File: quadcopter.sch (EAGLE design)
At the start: 61 parts, among them J1 ISP, J4 SIP-10_TH-254X10, M1 MOTOR_PADS, M2 MOTOR_PADS, M3 MOTOR_PADS, M4 MOTOR_PADS, U1 ATMEGA128RFA1, Y1 16MHz

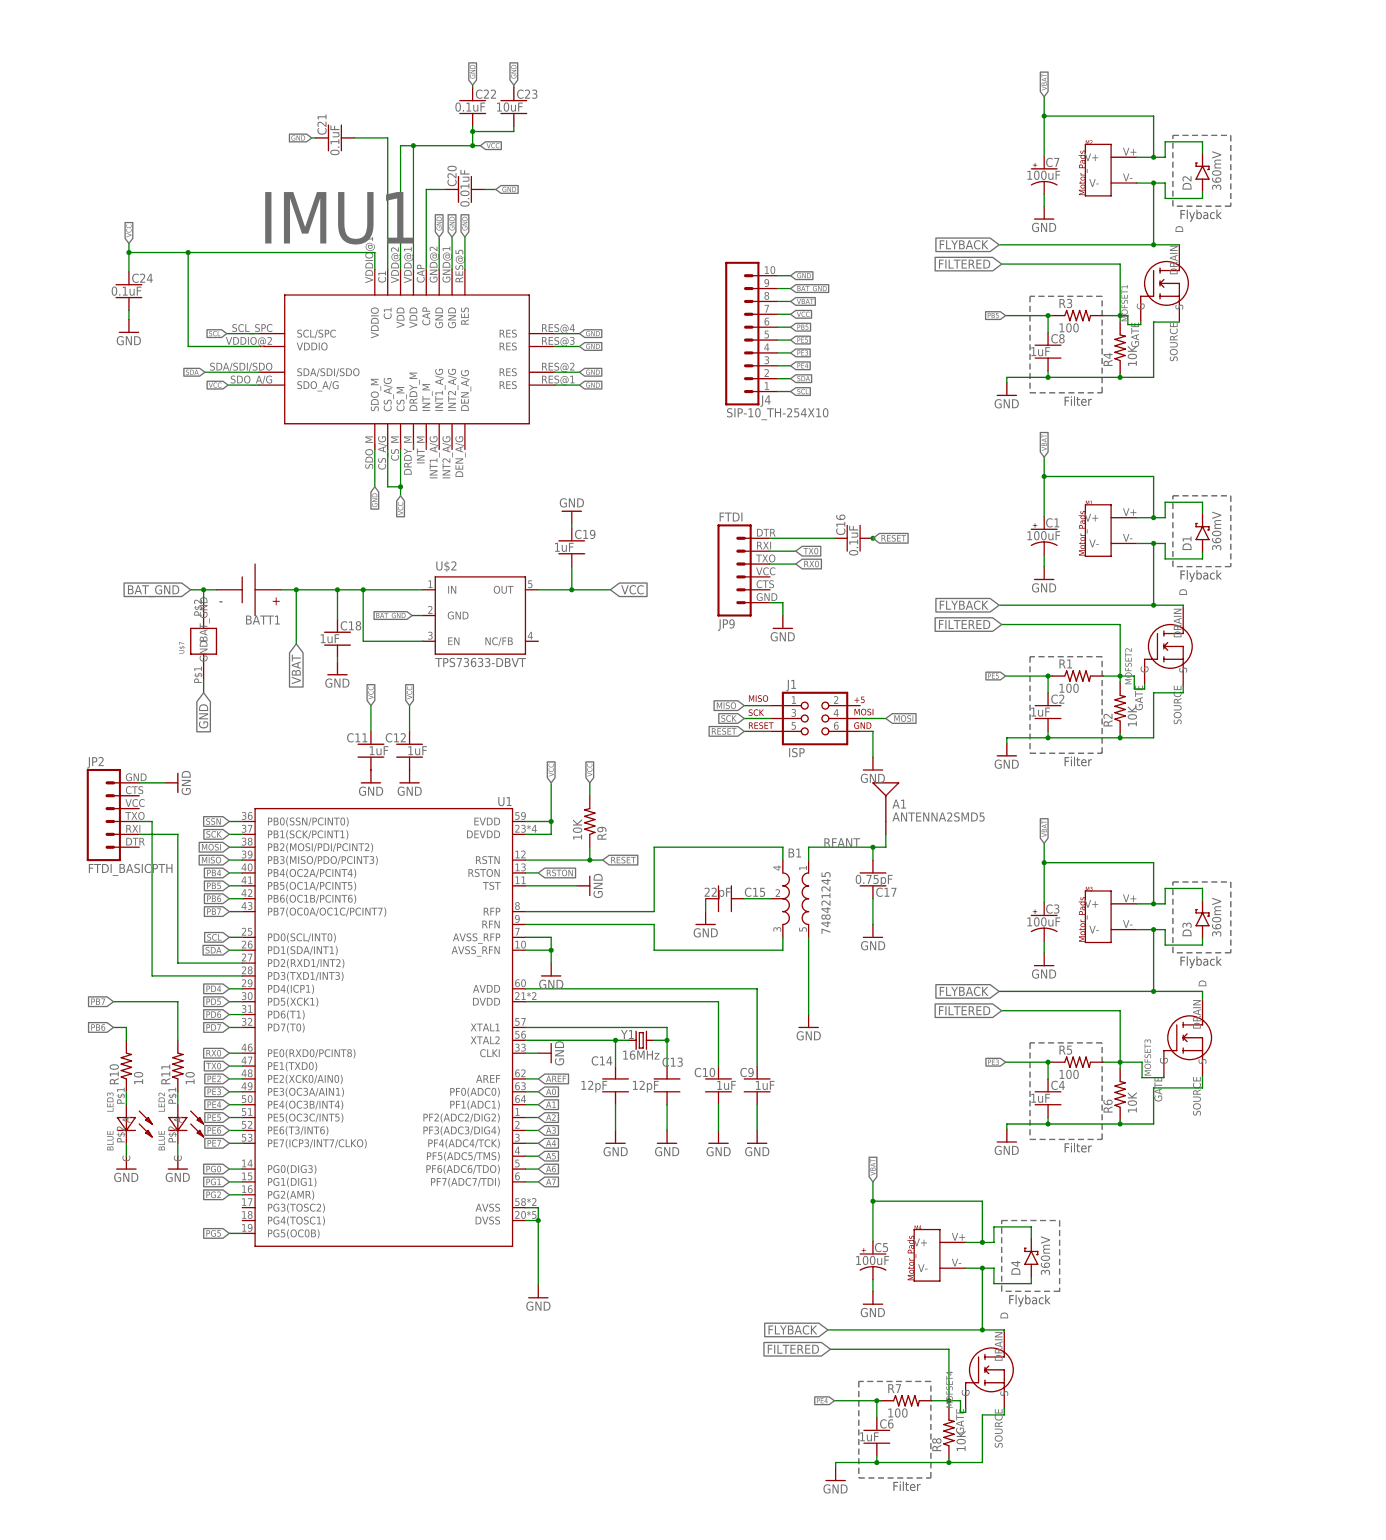
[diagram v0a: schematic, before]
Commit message: Schematic edited on April 24th
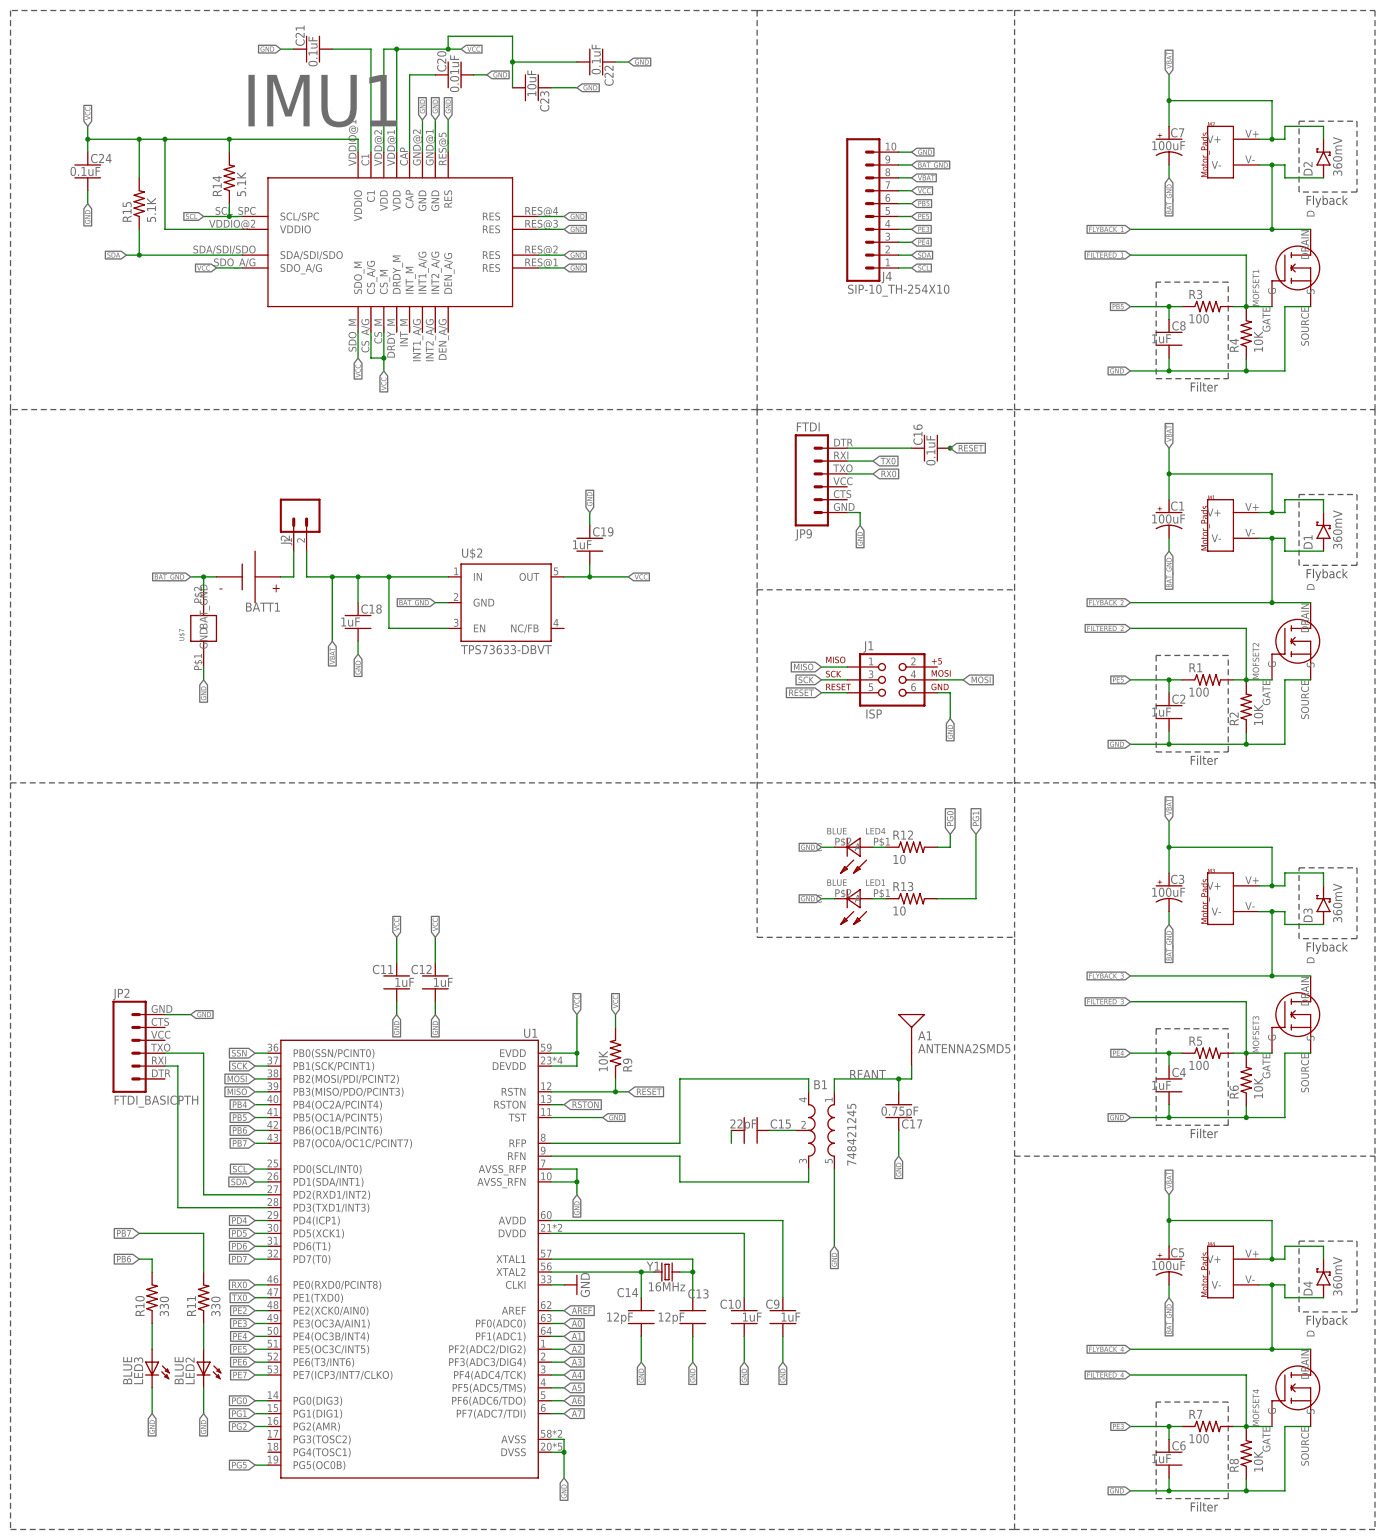
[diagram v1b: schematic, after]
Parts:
- added J2: (no value), quadparts:MALE_HEADER_2POS-2X1-0.1IN
- added LED1, LED4: BLUE, LEDs:LTST-C193TBKT-5ADISCRETE_LED
- added R12, R13: 10, quadparts_prebuilt:RESISTOR_SMD-2012-0805-10
- added R14, R15: 5.1K, quadparts_prebuilt:RESISTOR_SMD-2012-0805-5.1K
- LED2, LED3: device LEDs:LTST-C193TBKT-5ADISCRETE_LED -> Yueqi Wang-Lab2:LED5MM
- R10, R11: value 10 -> 330; device quadparts_prebuilt:RESISTOR_SMD-2012-0805-10 -> quadparts_prebuilt:RESISTOR_SMD-2012-0805-330
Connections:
- removed net FILTERED: MOFSET1.G, MOFSET2.G, MOFSET3.G, MOFSET4.G, R1.2, R2.2, R3.2, R4.2, R5.2, R6.2, R7.2, R8.2
- removed net FLYBACK: D1.A, D2.A, D3.A, D4.A, M1.V-, M2.V-, M3.V-, M4.V-, MOFSET1.D, MOFSET2.D, MOFSET3.D, MOFSET4.D
- removed net N$20: JP2.2, U1.PD2(RXD1/INT2)
- removed net N$21: JP2.3, U1.PD3(TXD1/INT3)
- new net FILTERED_1: MOFSET1.G, R3.2, R4.2
- new net FILTERED_2: MOFSET2.G, R1.2, R2.2
- new net FILTERED_3: MOFSET3.G, R5.2, R6.2
- new net FILTERED_4: MOFSET4.G, R7.2, R8.2
- new net FLYBACK_1: D2.A, M2.V-, MOFSET1.D
- new net FLYBACK_2: D1.A, M1.V-, MOFSET2.D
- new net FLYBACK_3: D3.A, M3.V-, MOFSET3.D
- new net FLYBACK_4: D4.A, M4.V-, MOFSET4.D
- new net N$24: C15.2
- new net N$3: LED4.A, R12.1
- new net N$4: JP2.2, U1.PD3(TXD1/INT3)
- new net N$5: JP2.3, U1.PD2(RXD1/INT2)
- new net N$6: LED1.A, R13.1
- new net N$7: BATT1.P, J2.1
- net BAT_GND: now also C1.-, C3.-, C5.-, C7.-
- net GND: now also LED1.C, LED4.C; no longer C1.-, C15.2, C3.-, C5.-, C7.-, IMU1.SDO_M
- net PE3: now also C6.1, R7.1; no longer C4.1, R5.1
- net PE4: now also C4.1, R5.1; no longer C6.1, R7.1
- net PG0: now also R12.2
- net PG1: now also R13.2
- net SCL: now also R14.1
- net SDA: now also R15.1
- net VBAT: now also J2.2; no longer BATT1.P
- net VCC: now also IMU1.SDO_M, R14.2, R15.2
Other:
- moved on the sheet: A1, B1, BATT1, C1, C10, C11, C12, C13, C14, C15, C16, C17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
